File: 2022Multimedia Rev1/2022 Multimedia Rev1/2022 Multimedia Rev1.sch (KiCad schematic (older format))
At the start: 37 parts, among them U1 TSR1-2433, U10 TSR1-2433, U2 TSR1-2433, U3 BDJ2GA5WEFJ, U4 TM4C129E_Launchpad, U5 TSR1-2433, U6 TSR1-2433, U7 TSR1-2433, U8 TSR1-2433, U9 TSR1-2433

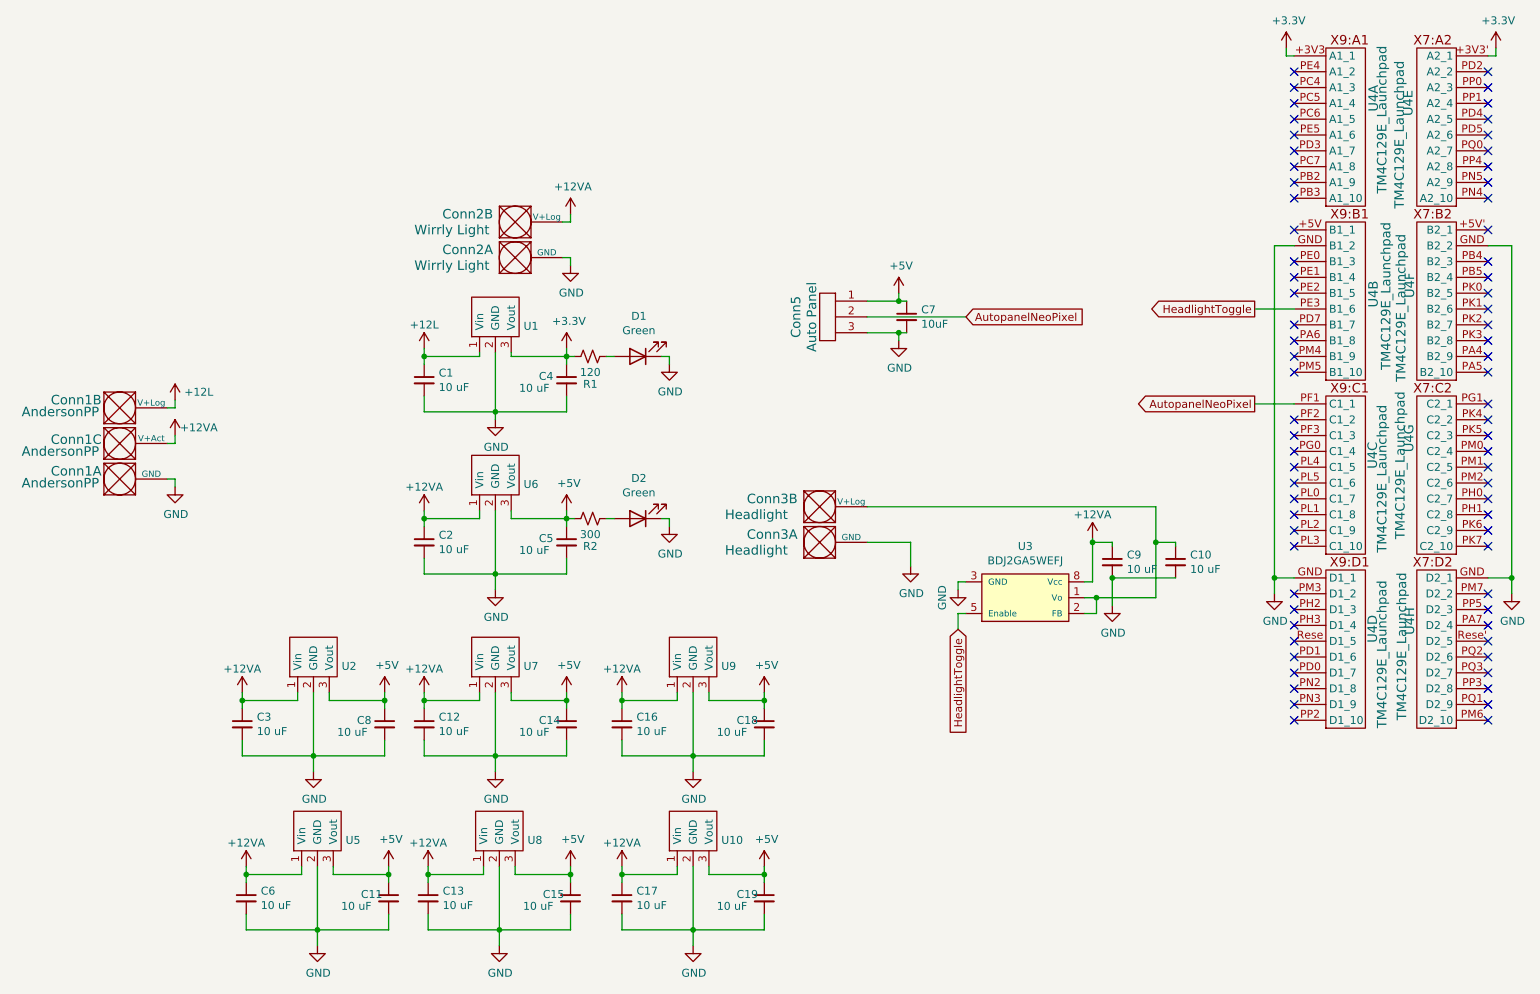
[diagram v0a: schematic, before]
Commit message: Finished rev2
gerbs and all, except bom
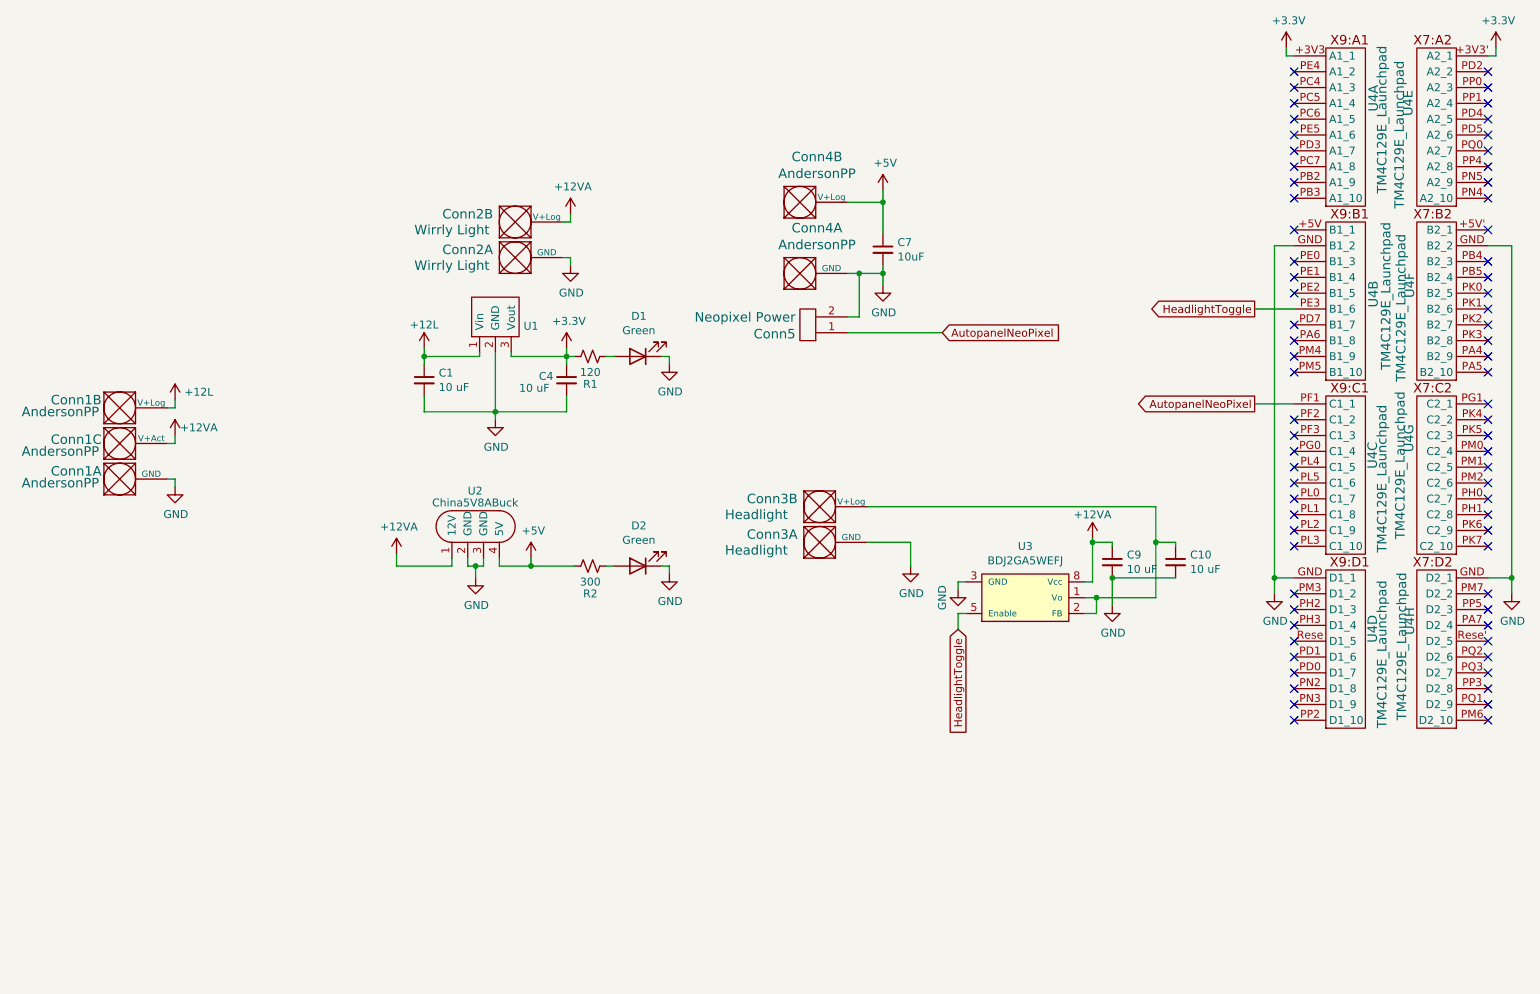
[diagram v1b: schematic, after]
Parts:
- removed C11, C12, C13, C14, C15, C16, C17, C18, C19, C2, C3, C5, C6, C8: 10 uF, Capacitor_SMD:C_0603_1608Metric_Pad1.05x0.95mm_HandSolder, symbol Device:C_Small
- removed Conn5: Auto Panel, MRDT_Connectors:MOLEX_uF_S_03_Horizontal, symbol MRDT_Connectors:Molex_uF_S_03
- removed U10, U2, U5, U6, U7, U8, U9: TSR1-2433, MRDT_Devices:TSR_1-2433, symbol MRDT_Devices:TSR1-2433
- added Conn4: AndersonPP, MRDT_Connectors:Square_Anderson_2_H_Side_By_Side, symbol MRDT_Connectors:AndersonPP
- added Conn5: Neopixel Power, MRDT_Connectors:MOLEX_uF_S_02_Horizontal, symbol MRDT_Connectors:Molex_uF_S_02
- added U2: China5V8ABuck, 2022 Multimedia Rev1:China5V8ABuck, symbol Multimedia_IC:China5V8ABuck
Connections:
- net +12VA: now also U2.1 (12V)
- net +5V: now also Conn4.2 (V+Log), U2.4 (5V)
- net AutopanelNeoPixel: now also Conn5.1
- net GND: now also Conn4.1 (GND), Conn5.2, U2.2 (GND), U2.3 (GND)
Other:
- moved on the sheet: C7, D2, R2
